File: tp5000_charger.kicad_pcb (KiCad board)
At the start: 2 copper layers, 41 x 30 mm, 23 parts, among them J1 VIN, J2 GND, J3 VOUT, J4 GND, J5 BAT+, J6 BAT-, P1 USB_C_Plug_USB2.0, U1 TP5000, U2 DW01, U3 FS8205A

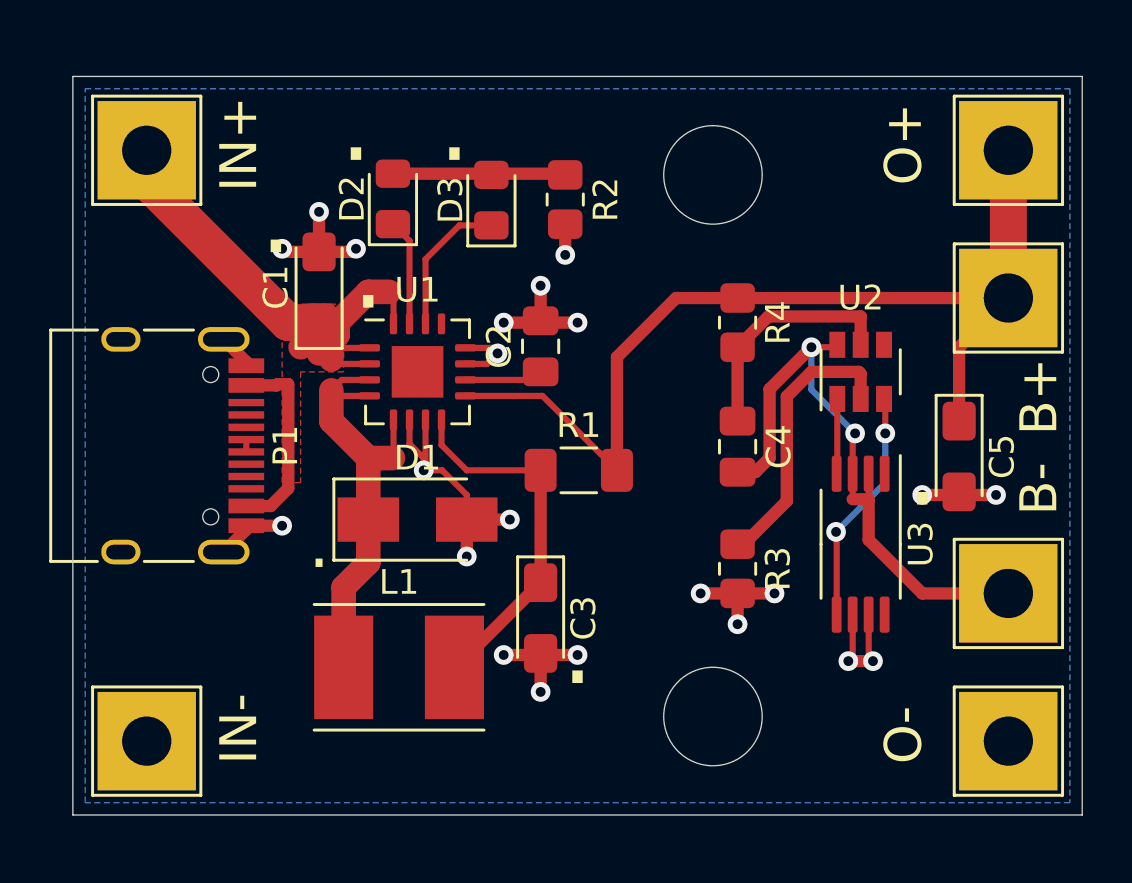
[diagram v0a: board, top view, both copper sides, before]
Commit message: pcb design V1.1
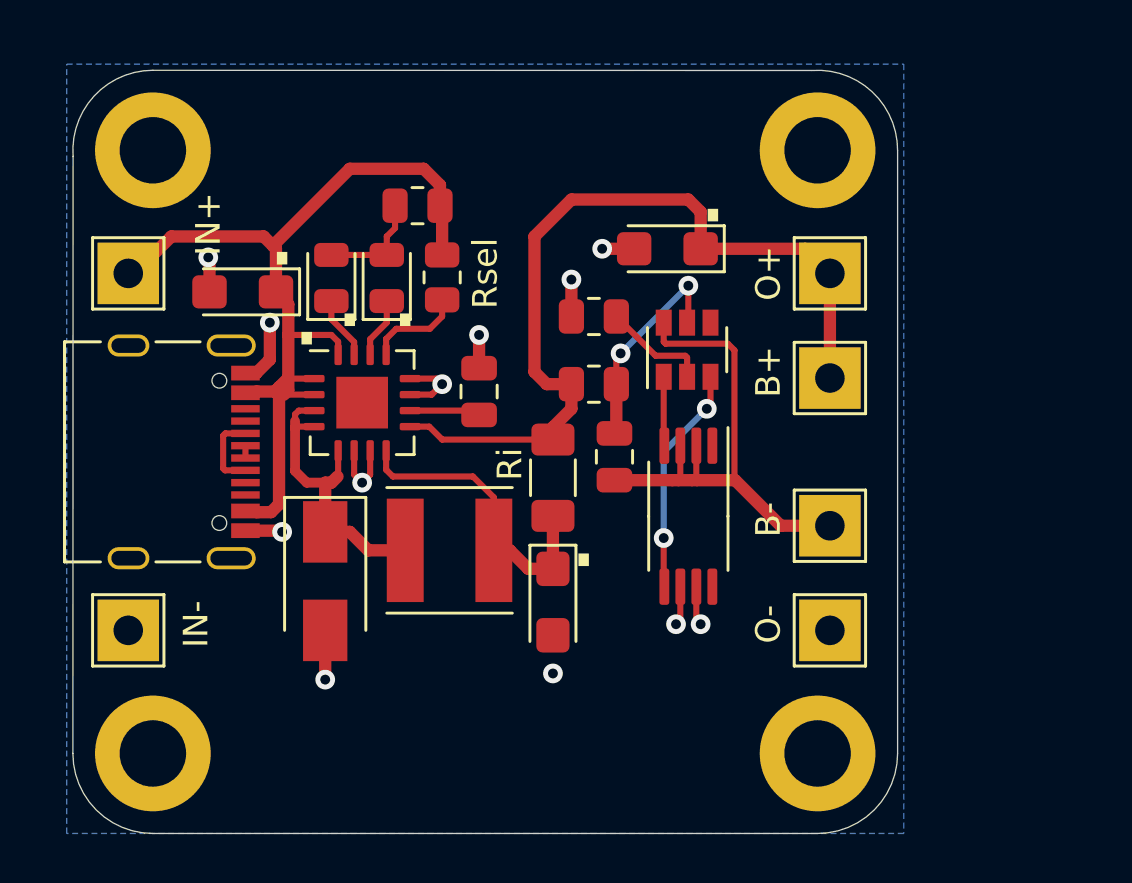
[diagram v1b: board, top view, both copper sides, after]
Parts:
- removed P1: USB_C_Plug_USB2.0, Connector_USB:USB_C_Receptacle_HRO_TYPE-C-31-M-12
- added H1: Mounting, MountingHole:MountingHole_2.7mm_M2.5_DIN965_Pad, F.Cu at (86.2, 110.0)
- added H2: Mounting, MountingHole:MountingHole_2.7mm_M2.5_DIN965_Pad, F.Cu at (86.2, 134.5)
- added H3: Mounting, MountingHole:MountingHole_2.7mm_M2.5_DIN965_Pad, F.Cu at (113.2, 110.0)
- added H4: Mounting, MountingHole:MountingHole_2.7mm_M2.5_DIN965_Pad, F.Cu at (113.2, 134.5)
- added J7: USB_C_Receptacle_USB2.0, Connector_USB:USB_C_Receptacle_Palconn_UTC16-G, F.Cu at (87.5, 122.2)
- added R5: 10k, Resistor_SMD:R_0805_2012Metric, F.Cu at (98.0, 115.2)
- C1, C3, C5: footprint Capacitor_Tantalum_SMD:CP_EIA-3216-12_Kemet-S_Pad1.58x1.35mm_HandSolder -> Capacitor_Tantalum_SMD:CP_EIA-3216-12_Kemet-S
- C2, C4: footprint Capacitor_SMD:C_0805_2012Metric_Pad1.18x1.45mm_HandSolder -> Capacitor_SMD:C_0805_2012Metric
- D2, D3: footprint LED_SMD:LED_0805_2012Metric_Pad1.15x1.40mm_HandSolder -> LED_SMD:LED_0805_2012Metric
- J1, J2, J3, J4, J5, J6: footprint TestPoint:TestPoint_THTPad_4.0x4.0mm_Drill2.0mm -> TestPoint:TestPoint_THTPad_2.5x2.5mm_Drill1.2mm
- L1: footprint Inductor_SMD:L_Taiyo-Yuden_NR-50xx_HandSoldering -> Inductor_SMD:L_Taiyo-Yuden_NR-50xx
- R2: value 10k -> 1k; footprint Resistor_SMD:R_0805_2012Metric_Pad1.20x1.40mm_HandSolder -> Resistor_SMD:R_0805_2012Metric
- R3, R4: footprint Resistor_SMD:R_0805_2012Metric_Pad1.20x1.40mm_HandSolder -> Resistor_SMD:R_0805_2012Metric
- moved C5 14.5 mm to (107.2, 114.0), turned to 180 degrees
- moved R3 11.8 mm to (104.2, 116.8), turned to 180 degrees
- moved J3 8.81 mm to (113.8, 115.0)
- moved J2 8.53 mm to (113.8, 129.5)
- moved J5 7.95 mm to (113.8, 119.2)
- moved J6 7.75 mm to (113.8, 125.2)
- moved U2 7.11 mm to (108.0, 118.1)
- moved U3 7.09 mm to (108.0, 124.9)
- moved R4 6.35 mm to (104.2, 119.5), turned to 0 degrees
- moved R2 6.01 mm to (97.0, 112.2), turned to 0 degrees
- moved D3 5.30 mm to (95.8, 115.2)
- moved L1 5.17 mm to (98.3, 126.2)
- moved J1 5.06 mm to (85.2, 115.0)
- moved C4 5.02 mm to (105.0, 122.5)
- moved J4 4.56 mm to (85.2, 129.5)
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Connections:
- R2 pad 2: GND -> VIN
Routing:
- net GND: track 45.4 -> 20.7 mm, vias 22 -> 12
- net Net-(R3-Pad1): track 11.4 -> 4.35 mm
- net VIN: track 30.8 -> 37.7 mm
- net B+: track 40.7 -> 34.8 mm
- net Net-(D1-Pad1): track 18.2 -> 12.6 mm
- net Net-(R5-Pad1): track 0.00 -> 3.97 mm
- net Net-(D3-Pad1): track 5.87 -> 2.45 mm
- net B-: track 24.7 -> 21.4 mm, vias 2 -> 0
- net Net-(J7-PadB6): track 0.00 -> 3.21 mm
- net Net-(D2-Pad2): track 7.02 -> 4.39 mm
- net Net-(C3-Pad1): track 15.0 -> 12.6 mm
- net Net-(D2-Pad1): track 4.33 -> 2.56 mm
- net Net-(C4-Pad1): track 9.67 -> 8.76 mm, vias 0 -> 2
- net Net-(P1-PadA6): track 0.50 -> 0.00 mm
- net Net-(J7-PadA6): track 0.00 -> 0.50 mm
- removed copper zone on F.Cu, net VIN
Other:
- board size 41 x 30 mm -> 33.5 x 31 mm
- board text added: "Ri"
- board text added: "Rsel"
- board text removed: "3.0V - 3.6V R1 1Ω100mA 0.2Ω500mA 0.1Ω1000mA"
- board text removed: "TP5000 LiFePo4 Charger"

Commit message: layout smaller
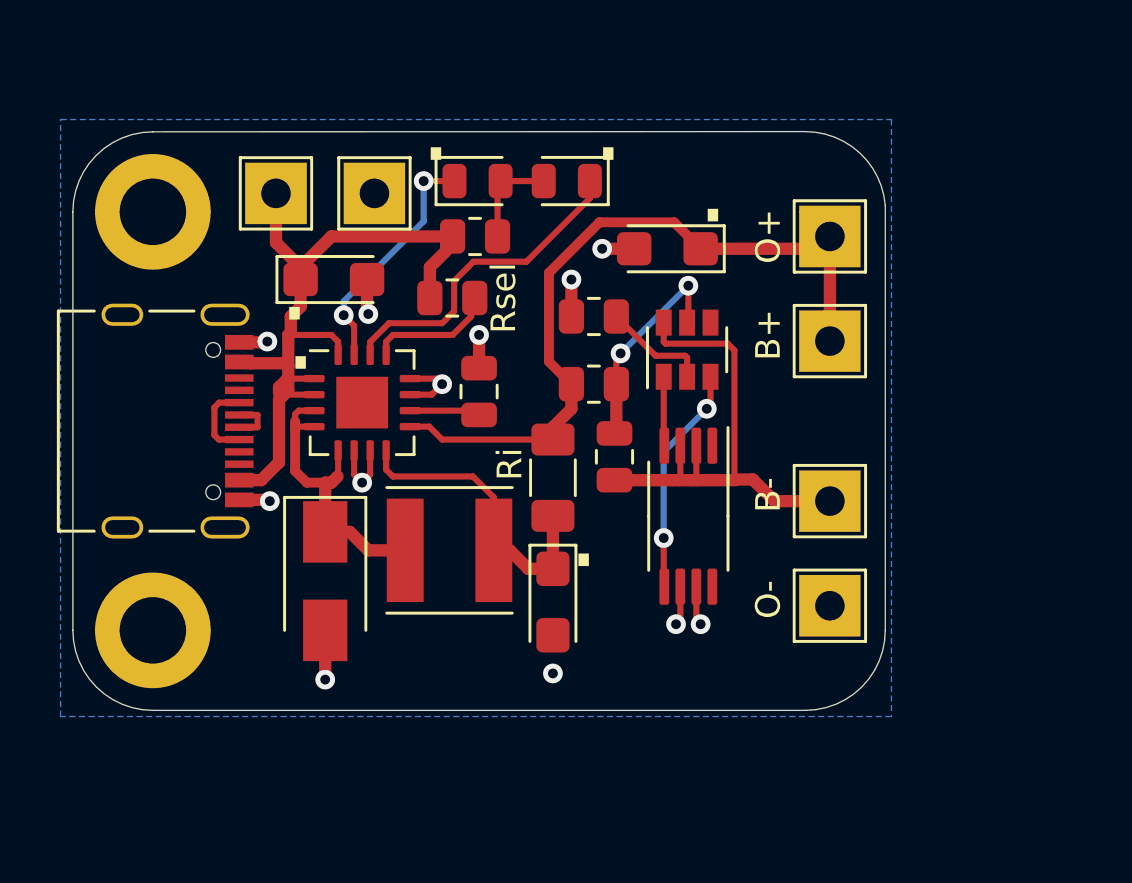
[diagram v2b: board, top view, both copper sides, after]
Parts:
- removed H3, H4: Mounting, MountingHole:MountingHole_2.7mm_M2.5_DIN965_Pad
- moved J4 20.4 mm to (95.2, 111.8)
- moved D3 8.31 mm to (103.1, 111.2), turned to 180 degrees
- moved D2 7.12 mm to (99.4, 111.2), turned to 0 degrees
- moved J1 6.82 mm to (91.2, 111.8)
- moved H2 5.00 mm to (86.2, 129.5)
- moved C1 3.73 mm to (93.6, 115.2), turned to 0 degrees
- moved R2 2.65 mm to (99.3, 113.5), turned to 180 degrees
- moved H1 2.50 mm to (86.2, 112.5)
- moved J3 1.50 mm to (113.8, 113.5)
- moved J5 1.50 mm to (113.8, 117.8)
- moved J7 1.27 mm to (87.2, 121.0)
- moved J2 1.00 mm to (113.8, 128.5)
- moved J6 1.00 mm to (113.8, 124.2)
- moved R5 0.93 mm to (98.4, 116.0), turned to 180 degrees
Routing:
- net Net-(D3-Pad1): track 2.45 -> 13.3 mm
- net Net-(D2-Pad1): track 2.56 -> 9.82 mm, vias 0 -> 2
- net VIN: track 37.7 -> 31.2 mm
- net B+: track 34.8 -> 32.1 mm
- net GND: track 20.7 -> 18.9 mm
- net Net-(J7-PadA6): track 0.50 -> 1.98 mm
- net Net-(R5-Pad1): track 3.97 -> 5.21 mm
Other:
- board size 33.5 x 31 mm -> 33 x 23.5 mm
- board text added: "Ri: 1=100mA 0.2=500mA 0.1=1000mA"
- board text added: "Rsel: 10k=4.2V open=3.6V"
- board text added: "TP5000 Lithium Charger V1.1"
